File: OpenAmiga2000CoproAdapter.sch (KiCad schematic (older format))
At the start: 23 parts, among them CN1 A2000_COPRO_SLOT, P1 CONN_2, P10 CONN_1, P11 CONN_1, P12 CONN_1, P13 CONN_1, P14 CONN_1, P15 CONN_1, P2 CONN_2, P3 CONN_2, P4 CONN_2, P5 CONN_1, P6 CONN_1, P7 CONN_1, P8 CONN_1, P9 CONN_1, U1 68000D, U10 Spare

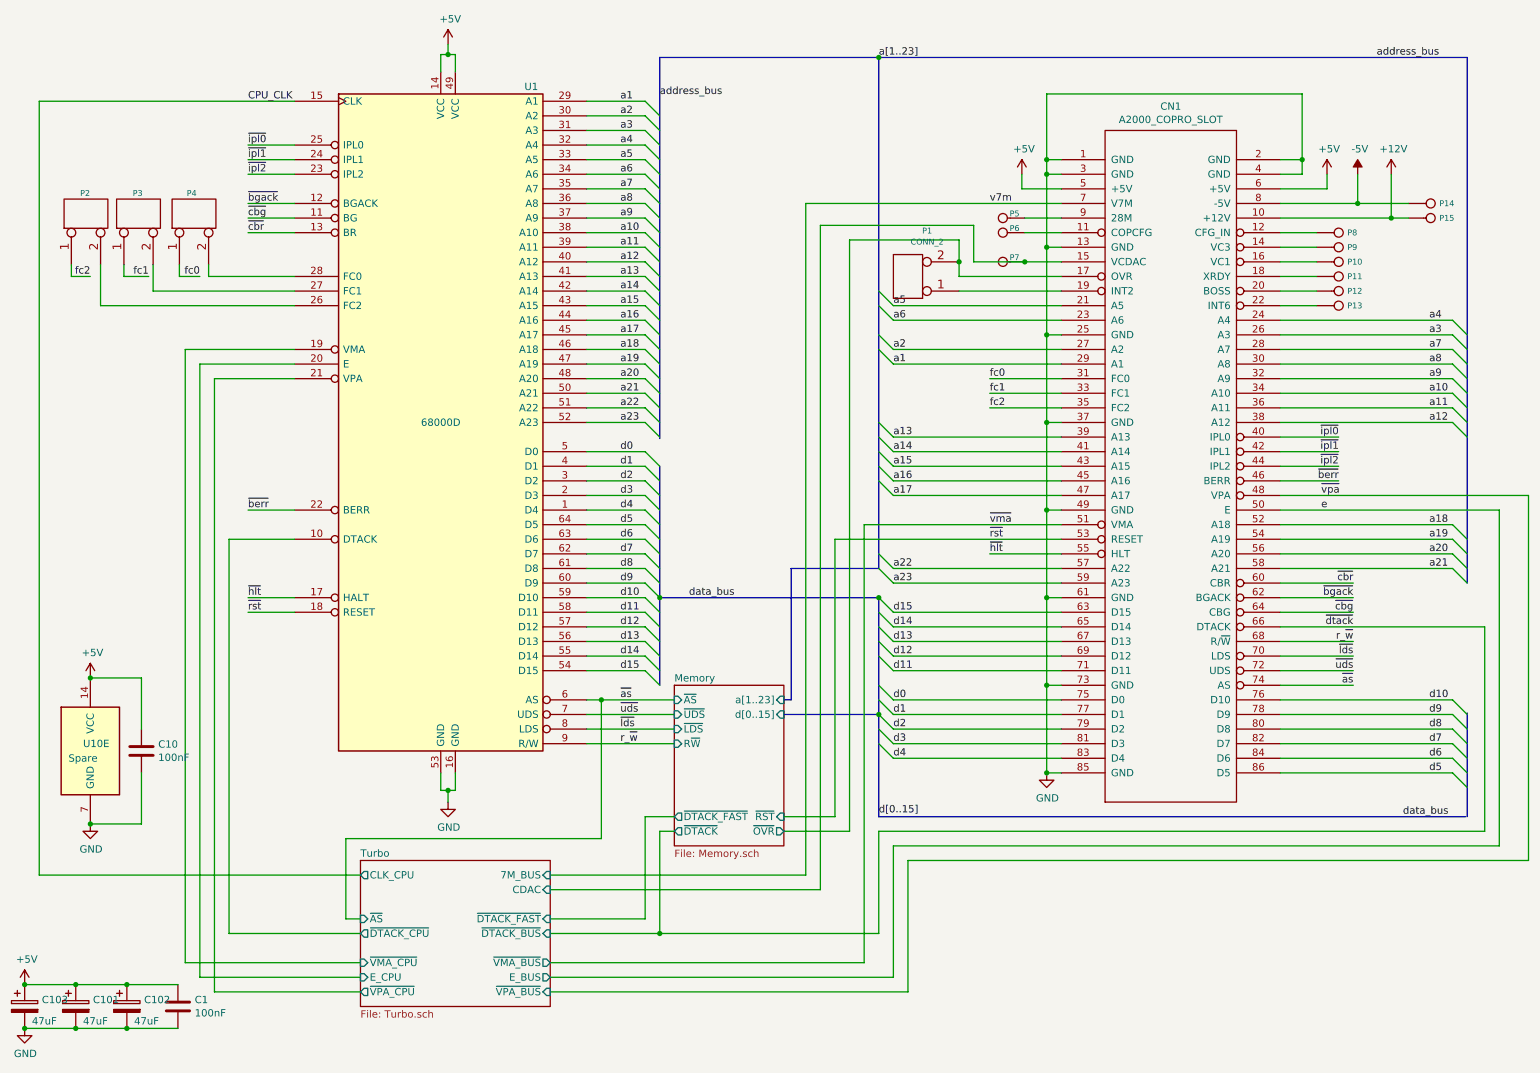
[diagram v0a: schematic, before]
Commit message: pins
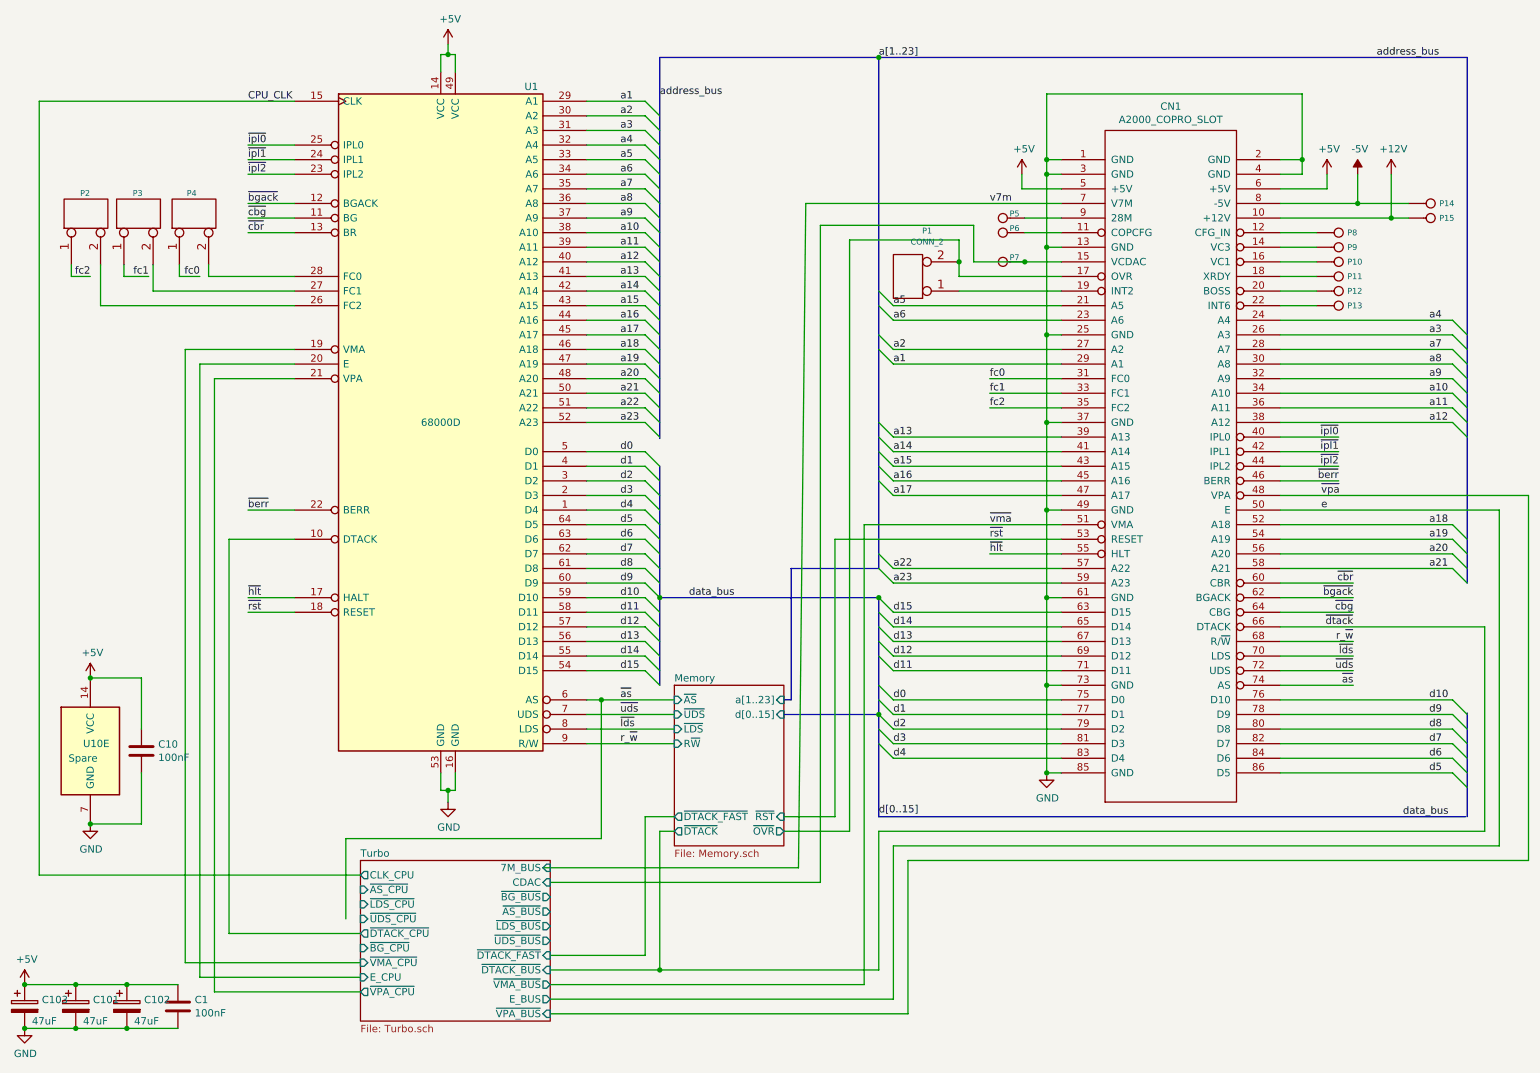
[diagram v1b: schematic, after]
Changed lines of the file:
@@
 Connection ~ 5000 4600
 $Sheet
-S 2950 6400 1300 1000
+S 2950 6400 1300 1100
 U 606B7AE6
 F0 "Turbo" 50
 F1 "Turbo.sch" 50
-F2 "7M_BUS" I R 4250 6500 50
-F3 "CDAC" I R 4250 6600 50
-F4 "~DTACK_BUS" I R 4250 6900 50
-F5 "~VPA_BUS" I R 4250 7300 50
-F6 "~AS" I L 2950 6800 50
-F7 "~VMA_BUS" O R 4250 7100 50
-F8 "~VPA_CPU" O L 2950 7300 50
-F9 "~DTACK_CPU" O L 2950 6900 50
-F10 "~DTACK_FAST" I R 4250 6800 50
-F11 "E_BUS" O R 4250 7200 50
-F12 "E_CPU" I L 2950 7200 50
-F13 "CLK_CPU" O L 2950 6500 50
-F14 "~VMA_CPU" I L 2950 7100 50
+F2 "7M_BUS" I R 4250 6450 50
+F3 "CDAC" I R 4250 6550 50
+F4 "~DTACK_BUS" I R 4250 7150 50
+F5 "~VPA_BUS" I R 4250 7450 50
+F6 "~VMA_BUS" O R 4250 7250 50
+F7 "~VPA_CPU" O L 2950 7300 50
+F8 "~DTACK_CPU" O L 2950 6900 50
+F9 "~DTACK_FAST" I R 4250 7050 50
+F10 "E_BUS" O R 4250 7350 50
+F11 "E_CPU" I L 2950 7200 50
+F12 "CLK_CPU" O L 2950 6500 50
+F13 "~VMA_CPU" I L 2950 7100 50
+F14 "~AS_CPU" I L 2950 6600 50
+F15 "~LDS_CPU" I L 2950 6700 50
+F16 "~UDS_CPU" I L 2950 6800 50
+F17 "~LDS_BUS" O R 4250 6850 50
+F18 "~UDS_BUS" O R 4250 6950 50
+F19 "~AS_BUS" O R 4250 6750 50
+F20 "~BG_CPU" I L 2950 7000 50
+F21 "~BG_BUS" O R 4250 6650 50
 $EndSheet
 Wire Wire Line
 	5100 6200 5000 6200
 Wire Wire Line
-	5000 6200 5000 6900
-Wire Wire Line
-	5000 6900 4250 6900
+	5000 6200 5000 7150
+Wire Wire Line
+	5000 7150 4250 7150
 Wire Wire Line
 	5100 6100 4900 6100
 Wire Wire Line
-	4900 6100 4900 6800
-Wire Wire Line
-	4900 6800 4250 6800
+	4900 6100 4900 7050
+Wire Wire Line
+	4900 7050 4250 7050
 Wire Bus Line
 	5850 5400 6500 5400
@@
 	7150 2300 7150 2050
 Wire Wire Line
-	6000 1900 6000 6500
-Wire Wire Line
-	4250 6600 6100 6600
+	6000 1900 5950 6450
+Wire Wire Line
+	4250 6550 6100 6550
 Wire Wire Line
 	10650 4800 10650 6200
@@
 	5900 4400 6500 4400
 Wire Wire Line
-	6000 6500 4250 6500
+	5950 6450 4200 6450
 Wire Wire Line
 	6200 6100 5850 6100
@@
 	6300 2150 6300 6200
 Wire Wire Line
-	6100 2050 6100 6600
+	6100 2050 6100 6550
 Wire Wire Line
 	6000 1900 7750 1900
@@
 	6400 4100 7750 4100
 Wire Wire Line
-	4250 7300 6700 7300
-Wire Wire Line
-	6700 7300 6700 6400
+	4250 7450 6700 7450
+Wire Wire Line
+	6700 7450 6700 6400
 Wire Wire Line
 	10950 6400 10950 3900
@@
 Wire Wire Line
 	1530 2500 2500 2500
-Wire Wire Line
-	2950 6800 2850 6800
 Wire Wire Line
 	2850 6800 2850 6250
@@
 	1950 3100 2500 3100
 Wire Wire Line
-	6400 4100 6400 7100
-Wire Wire Line
-	6600 6300 6600 7200
-Wire Wire Line
-	6400 7100 4250 7100
-Wire Wire Line
-	4250 7200 6600 7200
+	6400 4100 6400 7250
+Wire Wire Line
+	6600 6300 6600 7350
+Wire Wire Line
+	6400 7250 4250 7250
+Wire Wire Line
+	4250 7350 6600 7350
 Wire Wire Line
 	2950 7300 1950 7300
@@
 Connection ~ 650  7250
 Wire Wire Line
-	5000 6900 6500 6900
-Connection ~ 5000 6900
-Wire Wire Line
-	6500 6200 6500 6900
+	5000 7150 6500 7150
+Connection ~ 5000 7150
+Wire Wire Line
+	6500 6200 6500 7150
 Wire Wire Line
 	10750 6300 6600 6300
